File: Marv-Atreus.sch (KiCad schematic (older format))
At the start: 105 parts, among them SW1 SW_Push, U1 ATmega32U4-AU, Y1 16MHz

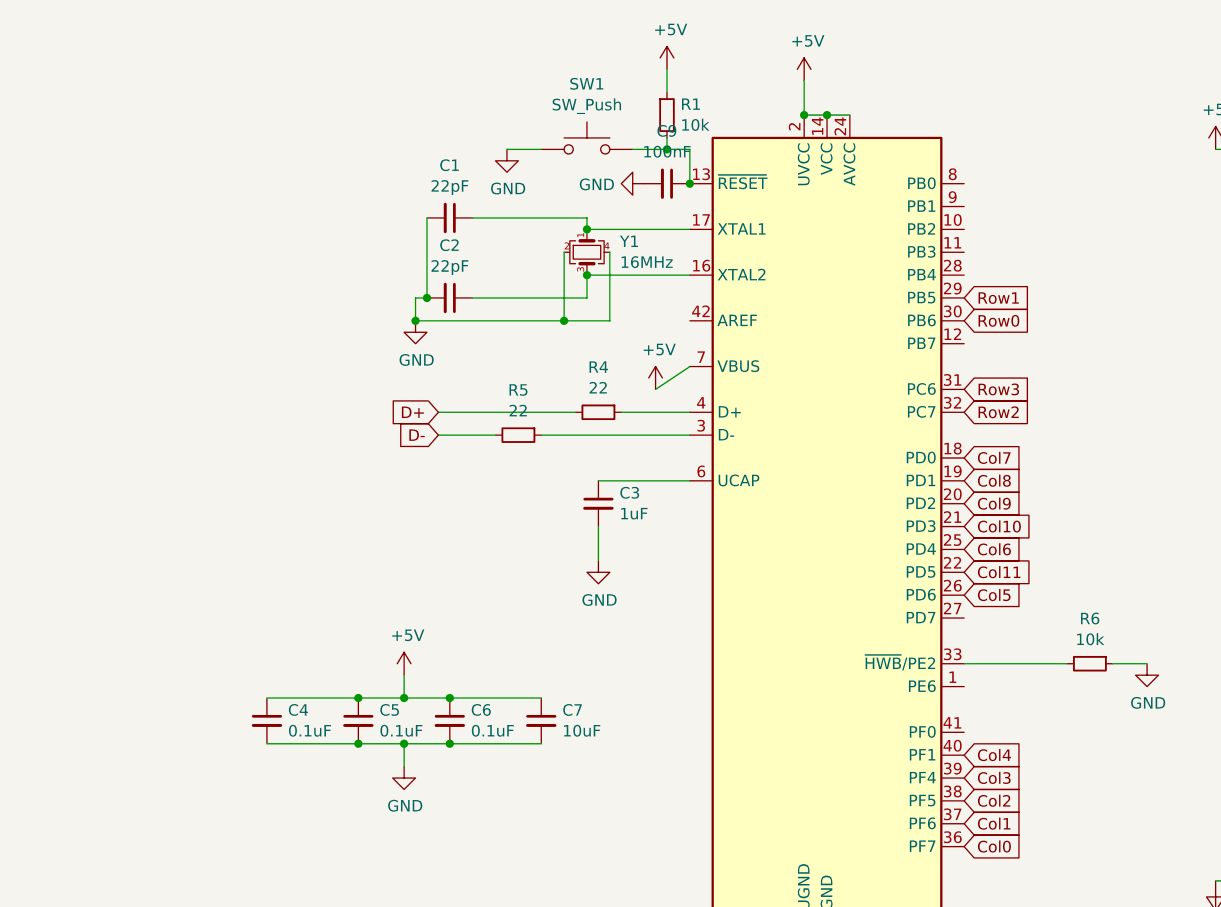
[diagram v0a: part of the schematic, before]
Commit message: Even more Updates
- switched from Crystal to resonator
- added ESD protection ic
- Cleaned up silkscreen
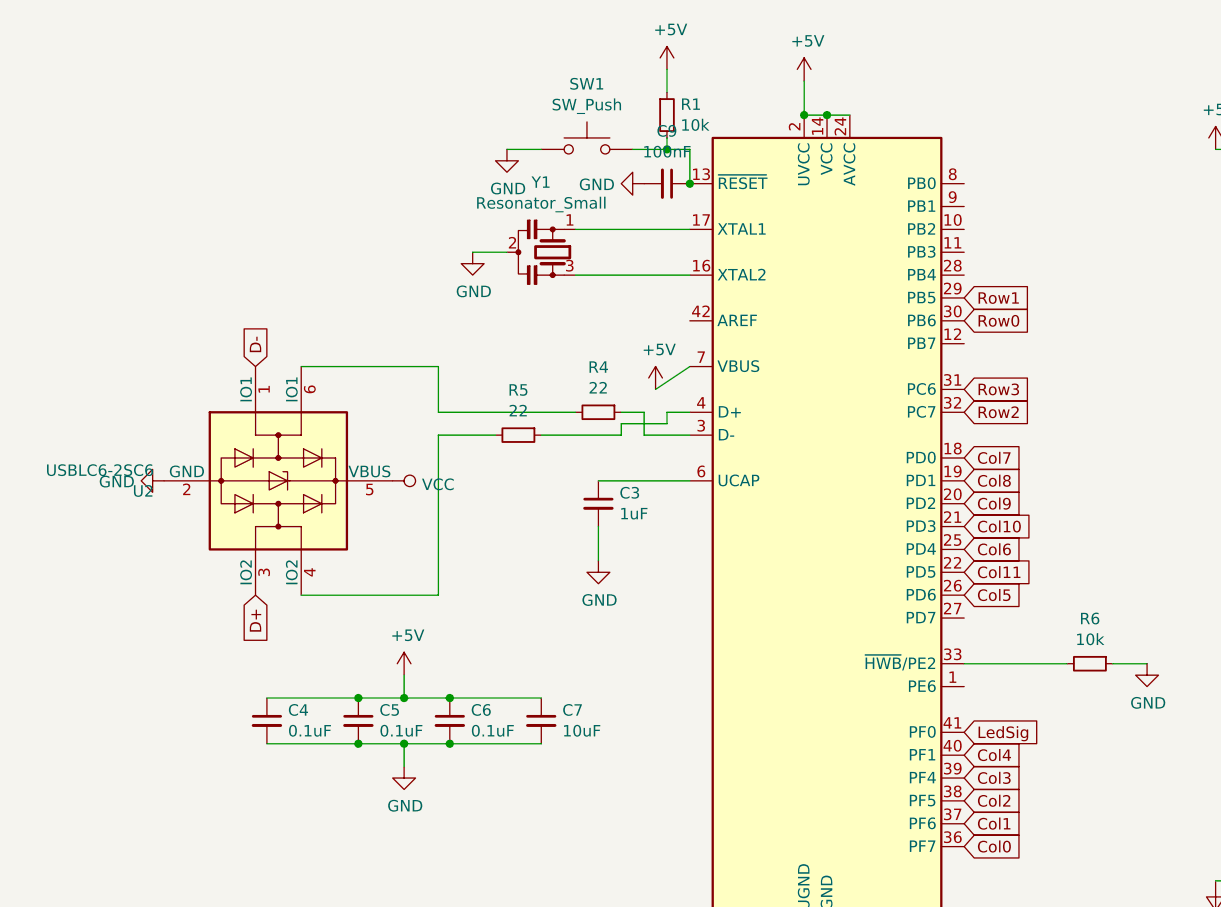
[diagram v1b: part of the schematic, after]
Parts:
- removed C1, C2: 22pF, Capacitor_SMD:C_0603_1608Metric, symbol Device:C_Small
- removed Y1: 16MHz, Crystal:Crystal_SMD_3225-4Pin_3.2x2.5mm, symbol Device:Crystal_GND24_Small
- added U2: USBLC6-2SC6, Package_TO_SOT_SMD:SOT-23-6, symbol Power_Protection:USBLC6-2SC6
- added Y1: Resonator_Small, Crystal:Resonator_SMD_muRata_CSTxExxV-3Pin_3.0x1.1mm, symbol Device:Resonator_Small
- D1, D10, D11, D12, D13, D14, D15, D16, D17, D18, D19, D2, D20, D21, D22, D23, D24, D25, D28, D29, D3, D30, D31, D32, D33, D34, D35, D36, D37, D38, D39, D4, D40, D41, D42, D43, D44, D5, D6, D7, D8, D9: footprint Diode_SMD:D_SOD-123 -> random-keyboard-parts:D_SOD-123_NoReference
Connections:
- net D+: now also U2.3 (IO2); no longer R4.2
- net D-: now also U2.1 (IO1); no longer R5.2
- net GND: now also U2.2 (GND), Y1.2
- net VCC: now also U2.5 (VBUS)
- net at U1.16 (XTAL2): now also Y1.3
- net at U1.17 (XTAL1): now also Y1.1
- net at U1.3 (D-): now also R4.1; no longer R5.1
- net at U1.4 (D+): now also R5.1; no longer R4.1
- net LedSig: now reaches U1.41 (PF0)
- new net: R4.2, U2.6 (IO1)
- new net: R5.2, U2.4 (IO2)
